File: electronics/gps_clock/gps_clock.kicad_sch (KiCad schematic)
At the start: 28 parts, among them J1 USB_C_Receptacle_PowerOnly_24P, J2 TC2030, SW1 SW_Push, U1 MIC5365-3.3YD5, U2 PA1616D, U3 STM32G070RBTx, X1 32kHz768

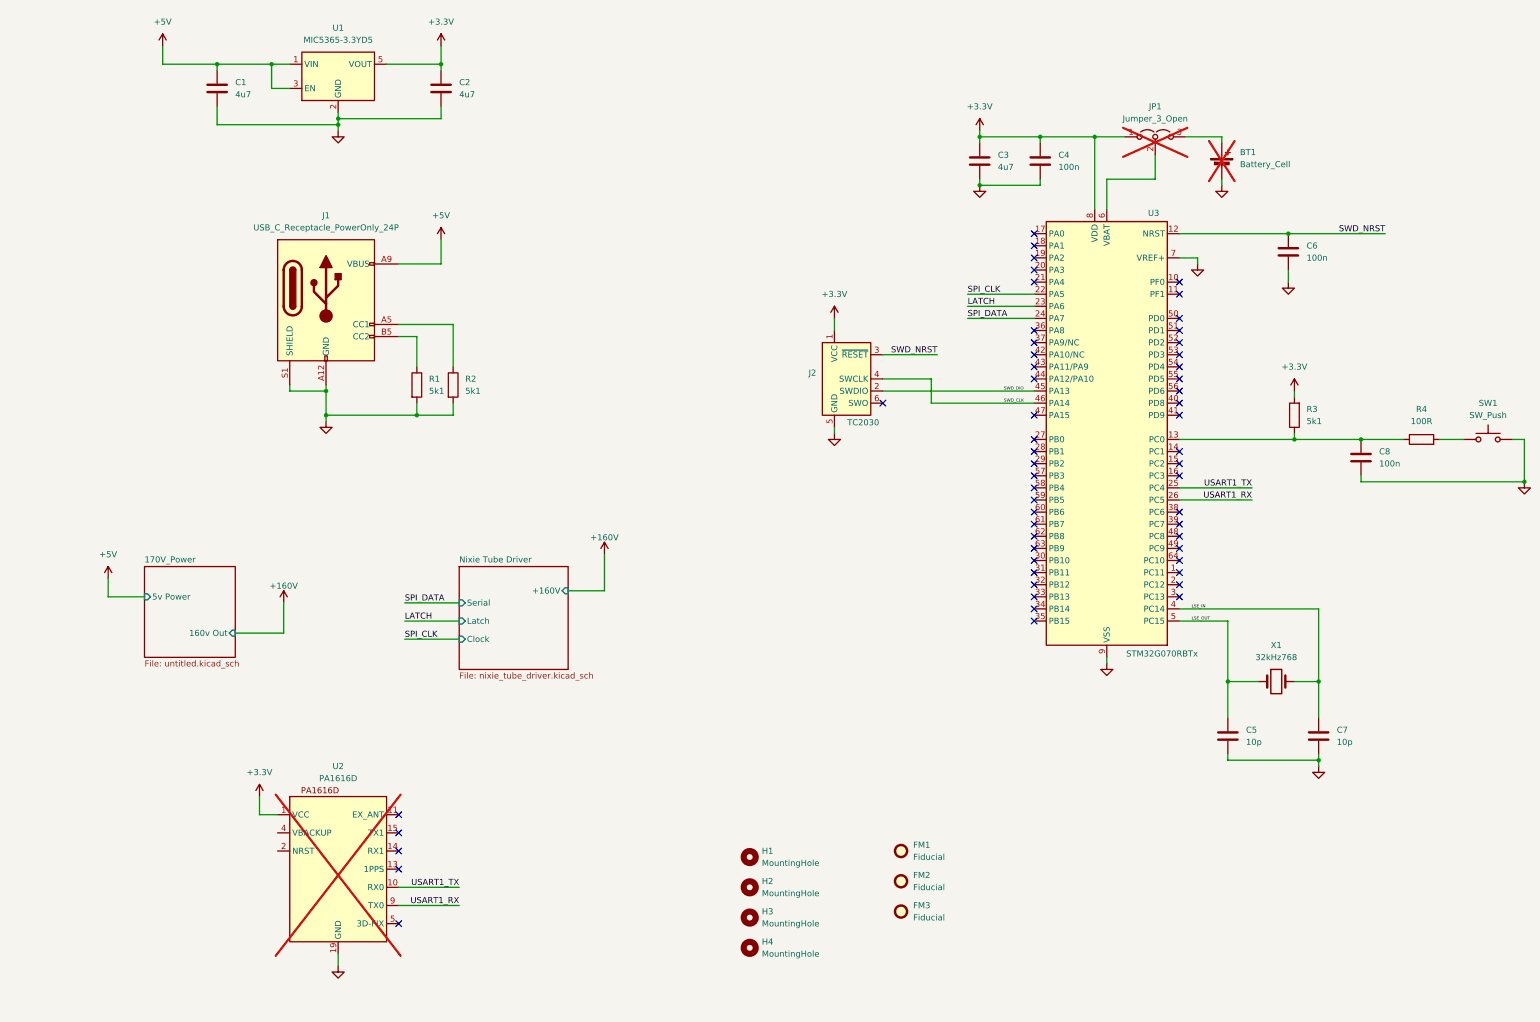
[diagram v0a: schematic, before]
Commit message: updated pcb
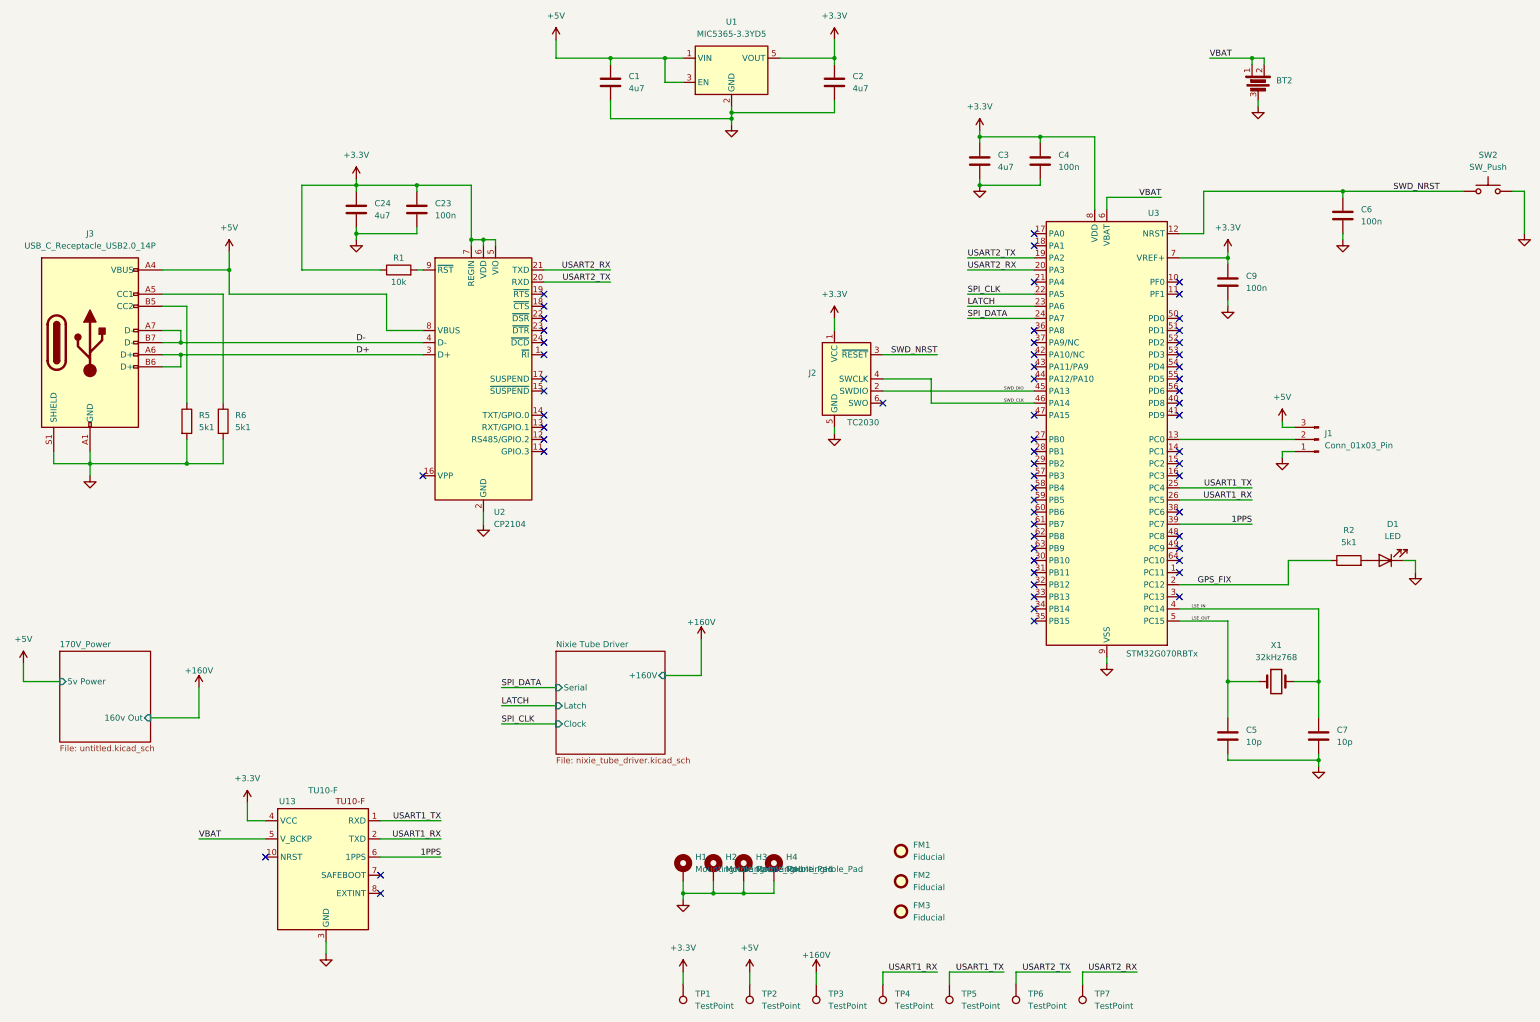
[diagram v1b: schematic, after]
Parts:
- removed BT1: Battery_Cell, Library:MS518SE-FL35E, symbol Device:Battery_Cell
- removed C8: 100n, Capacitor_SMD:C_0402_1005Metric, symbol Device:C
- removed H1, H2, H3, H4: MountingHole, MountingHole:MountingHole_5mm_Pad_Via, symbol Mechanical:MountingHole
- removed J1: USB_C_Receptacle_PowerOnly_24P, Connector_USB:USB_C_Receptacle_XKB_U262-16XN-4BVC11, symbol Connector:USB_C_Receptacle_PowerOnly_24P
- removed JP1: Jumper_3_Open, Connector_PinHeader_2.54mm:PinHeader_1x03_P2.54mm_Vertical, symbol Jumper:Jumper_3_Open
- removed R3: 5k1, Resistor_SMD:R_0402_1005Metric, symbol Device:R
- removed R4: 100R, Resistor_SMD:R_0402_1005Metric, symbol Device:R
- removed SW1: SW_Push, Button_Switch_SMD:SW_Push_1P1T_XKB_TS-1187A, symbol Switch:SW_Push
- removed U2: PA1616D, Library:CD-PA1616D_ADA, symbol NixieTubeClock:PA1616D
- added BT2: ~, Library:BAT-SMD_MY-1220-03, symbol CustomLibrary:Multi_Prong_Battery_Cell
- added C23, C9: 100n, Capacitor_SMD:C_0402_1005Metric, symbol Device:C
- added C24: 4u7, Capacitor_SMD:C_0603_1608Metric, symbol Device:C
- added D1: LED, Diode_SMD:D_0603_1608Metric, symbol Device:LED
- added H1, H2, H3, H4: MountingHole_Pad, MountingHole:MountingHole_3mm_Pad_Via, symbol Mechanical:MountingHole_Pad
- added J1: Conn_01x03_Pin, Connector_Molex:Molex_PicoBlade_53261-0371_1x03-1MP_P1.25mm_Horizontal, symbol Connector:Conn_01x03_Pin
- added J3: USB_C_Receptacle_USB2.0_14P, Library:USB-C-SMD_U263-241N-4BQC02, symbol Connector:USB_C_Receptacle_USB2.0_14P
- added R5, R6: 5k1, Resistor_SMD:R_0402_1005Metric, symbol Device:R
- added SW2: SW_Push, Button_Switch_SMD:SW_Push_1P1T_XKB_TS-1187A, symbol Switch:SW_Push
- added TP1, TP2, TP3, TP4, TP5, TP6, TP7: TestPoint, TestPoint:TestPoint_Pad_D2.5mm, symbol Connector:TestPoint
- added U13: TU10-F, Library:TU10-F, symbol NixieTubeClock:TU10-F
- added U2: CP2104, Package_DFN_QFN:QFN-24-1EP_4x4mm_P0.5mm_EP2.7x2.7mm, symbol Interface_USB:CP2104
- R1: value 5k1 -> 10k
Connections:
- net +160V: now also TP3.1
- net +3.3V: now also R1.1, U3.7 (VREF+), C23.1, C24.1, C9.1, TP1.1, U13.4 (VCC), U2.5 (VIO), U2.6 (VDD), U2.7 (REGIN)
- net +5V: now also J1.3 (Pin_3), J3.A4 (VBUS), J3.A9 (VBUS), J3.B4 (VBUS), J3.B9 (VBUS), TP2.1, U2.8 (VBUS)
- net GND: now also BT2.3, C23.2, C24.2, C9.2, D1.1 (K), H1.1, H2.1, H3.1, H4.1, J1.1 (Pin_1), J3.A1 (GND), J3.A12 (GND), J3.B1 (GND), J3.B12 (GND), J3.S1 (SHIELD), R5.2, R6.2, SW2.2, U13.12 (GND), U13.3 (GND), U2.2 (GND), U2.25 (GND); no longer R1.2, R2.2, U3.7 (VREF+)
- net SWD_NRST: now also SW2.1
- net USART1_RX: now also TP4.1, U13.2 (TXD)
- net USART1_TX: now also TP5.1, U13.1 (RXD)
- net at U3.13 (PC0): now also J1.2 (Pin_2)
- net GPS_FIX: now reaches R2.1
- net GPS_FIX: now also U3.2 (PC12)
- net USART2_TX: now reaches U3.19 (PA2)
- net USART2_TX: now also TP6.1, U2.20 (RXD)
- net USART2_RX: now reaches U3.20 (PA3)
- net USART2_RX: now also TP7.1, U2.21 (TXD)
- net 1PPS: now reaches U3.39 (PC7)
- net 1PPS: now also U13.6 (1PPS)
- net VBAT: now reaches U3.6 (VBAT)
- net VBAT: now also BT2.1, BT2.2, U13.5 (V_BCKP)
- new net: R1.2, U2.9 (~{RST})
- new net: D1.2 (A), R2.2
- new net: J3.B5 (CC2), R5.1
- new net: J3.A5 (CC1), R6.1
- new net D+: J3.A6 (D+), J3.B6 (D+), U2.3 (D+)
- new net D-: J3.A7 (D-), J3.B7 (D-), U2.4 (D-)
- no-connect marks 55 -> 62
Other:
- moved on the sheet: C1, C2, C6, U1
